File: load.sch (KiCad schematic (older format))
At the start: 28 parts, among them J1 Load +, J2 Load -, Q1 IRFZ44N, Q2 IRFZ44N, Q3 IRFZ44N, Q4 IRFZ44N, U1 LM358, U2 LM7805_TO220, U3 MCP1525-TO

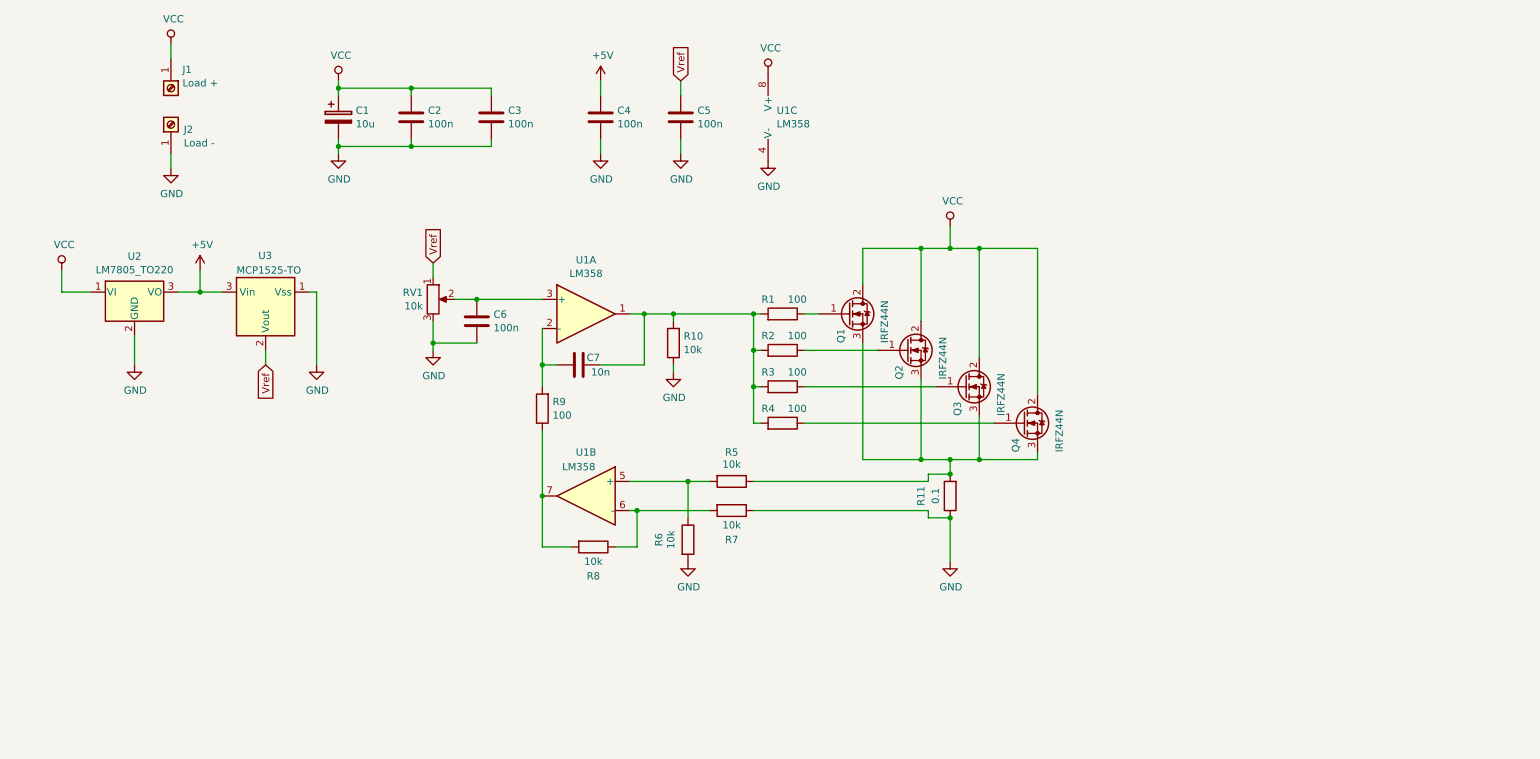
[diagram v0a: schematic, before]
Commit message: almost
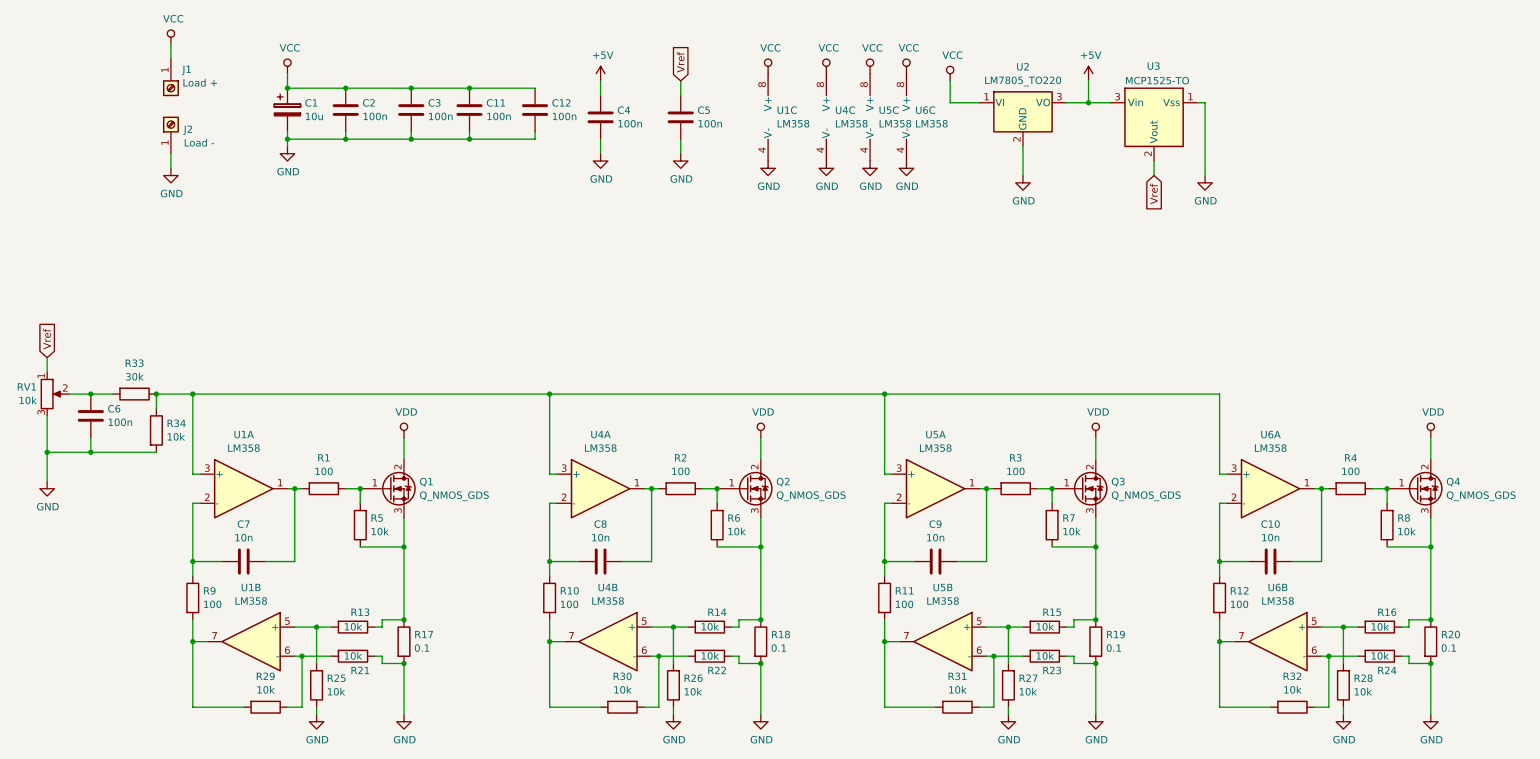
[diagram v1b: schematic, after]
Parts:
- added C10, C8, C9: 10n, Capacitor_SMD:C_0805_2012Metric_Pad1.15x1.40mm_HandSolder, symbol Device:C
- added C11, C12: 100n, Capacitor_SMD:C_0805_2012Metric_Pad1.15x1.40mm_HandSolder, symbol Device:C
- added R12: 100, Resistor_SMD:R_0805_2012Metric_Pad1.15x1.40mm_HandSolder, symbol Device:R
- added R13, R14, R15, R16, R21, R22, R23, R24, R25, R26, R27, R28, R29, R30, R31, R32, R34: 10k, Resistor_SMD:R_0805_2012Metric_Pad1.15x1.40mm_HandSolder, symbol Device:R
- added R17, R18, R19, R20: 0.1, Resistor_THT:R_Axial_DIN0922_L20.0mm_D9.0mm_P30.48mm_Horizontal, symbol Device:R
- added R33: 30k, Resistor_SMD:R_0805_2012Metric_Pad1.15x1.40mm_HandSolder, symbol Device:R
- added U4, U5, U6: LM358, Package_SO:SO-8_5.3x6.2mm_P1.27mm, symbol Amplifier_Operational:LM358
- C1: footprint Capacitor_THT:CP_Radial_D4.0mm_P2.00mm -> Capacitor_SMD:C_0805_2012Metric_Pad1.15x1.40mm_HandSolder
- C2, C3, C4, C5, C6, C7: footprint Capacitor_THT:C_Disc_D5.0mm_W2.5mm_P2.50mm -> Capacitor_SMD:C_0805_2012Metric_Pad1.15x1.40mm_HandSolder
- Q1, Q2, Q3, Q4: value IRFZ44N -> Q_NMOS_GDS
- R1, R2, R3, R4, R5, R6, R8, R9: footprint Resistor_THT:R_Axial_DIN0207_L6.3mm_D2.5mm_P2.54mm_Vertical -> Resistor_SMD:R_0805_2012Metric_Pad1.15x1.40mm_HandSolder
- R10: value 10k -> 100; footprint Resistor_THT:R_Axial_DIN0207_L6.3mm_D2.5mm_P2.54mm_Vertical -> Resistor_SMD:R_0805_2012Metric_Pad1.15x1.40mm_HandSolder
- R11: value 0.1 -> 100; footprint Resistor_THT:R_Axial_DIN0207_L6.3mm_D2.5mm_P2.54mm_Vertical -> Resistor_SMD:R_0805_2012Metric_Pad1.15x1.40mm_HandSolder
- R7: footprint Resistor_THT:R_Axial_DIN0207_L6.3mm_D2.5mm_P10.16mm_Horizontal -> Resistor_SMD:R_0805_2012Metric_Pad1.15x1.40mm_HandSolder
- RV1: footprint Potentiometer_THT:Potentiometer_Bourns_3266W_Vertical -> Potentiometer_THT:Potentiometer_Alps_RK097_Single_Horizontal
- U1: footprint Package_DIP:DIP-8_W7.62mm -> Package_SO:SO-8_5.3x6.2mm_P1.27mm
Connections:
- net GND: now also C11.2, C12.2, R17.2, R18.2, R19.2, R20.2, R21.1, R22.1, R23.1, R24.1, R25.1, R26.1, R27.1, R28.1, R34.2, U4.4 (V-), U5.4 (V-), U6.4 (V-); no longer R10.1, R11.1, R6.2, R7.1
- net VCC: now also C11.1, C12.1, U4.8 (V+), U5.8 (V+), U6.8 (V+); no longer Q1.2 (D), Q2.2 (D), Q3.2 (D), Q4.2 (D)
- net at C7.2, U1.2 (-): now also R9.1; no longer R9.2
- net at C6.1, RV1.2: now also R33.2; no longer U1.3 (+)
- net at Q1.1 (G), R1.1: now also R5.2
- net at Q2.1 (G), R2.1: now also R6.2
- net at Q3.1 (G), R3.1: now also R7.2
- net at Q4.1 (G), R4.1: now also R8.2
- new net: Q4.3 (S), R16.1, R20.1, R8.1
- new net: C10.2, R12.1, U6.2 (-)
- new net: R12.2, R32.2, U6.7
- new net: C10.1, R4.2, U6.1
- new net: R33.1, R34.1, U1.3 (+), U4.3 (+), U5.3 (+), U6.3 (+)
- new net: R16.2, R28.2, U6.5 (+)
- new net: R24.2, R32.1, U6.6 (-)
- new net: Q3.3 (S), R15.1, R19.1, R7.1
- new net: C9.2, R11.1, U5.2 (-)
- new net: R11.2, R31.2, U5.7
- new net: C9.1, R3.2, U5.1
- new net: R15.2, R27.2, U5.5 (+)
- new net: R23.2, R31.1, U5.6 (-)
- new net: Q2.3 (S), R14.1, R18.1, R6.1
- new net: C8.2, R10.1, U4.2 (-)
- new net: R10.2, R30.2, U4.7
- new net: C8.1, R2.2, U4.1
- new net: R14.2, R26.2, U4.5 (+)
- new net: R22.2, R30.1, U4.6 (-)
- new net: Q1.3 (S), R13.1, R17.1, R5.1
- new net: R29.2, R9.2, U1.7
- new net: C7.1, R1.2, U1.1
- new net: R13.2, R25.2, U1.5 (+)
- new net: R21.2, R29.1, U1.6 (-)
- new net VDD: Q1.2 (D), Q2.2 (D), Q3.2 (D), Q4.2 (D)
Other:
- moved on the sheet: C1, C2, C3, C6, RV1, U2, U3
